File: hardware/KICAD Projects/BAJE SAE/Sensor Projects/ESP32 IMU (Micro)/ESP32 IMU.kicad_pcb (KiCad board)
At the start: 2 copper layers, 57.1 x 72 mm, 12 parts, among them J1 +5V, U1 BA50JC5T

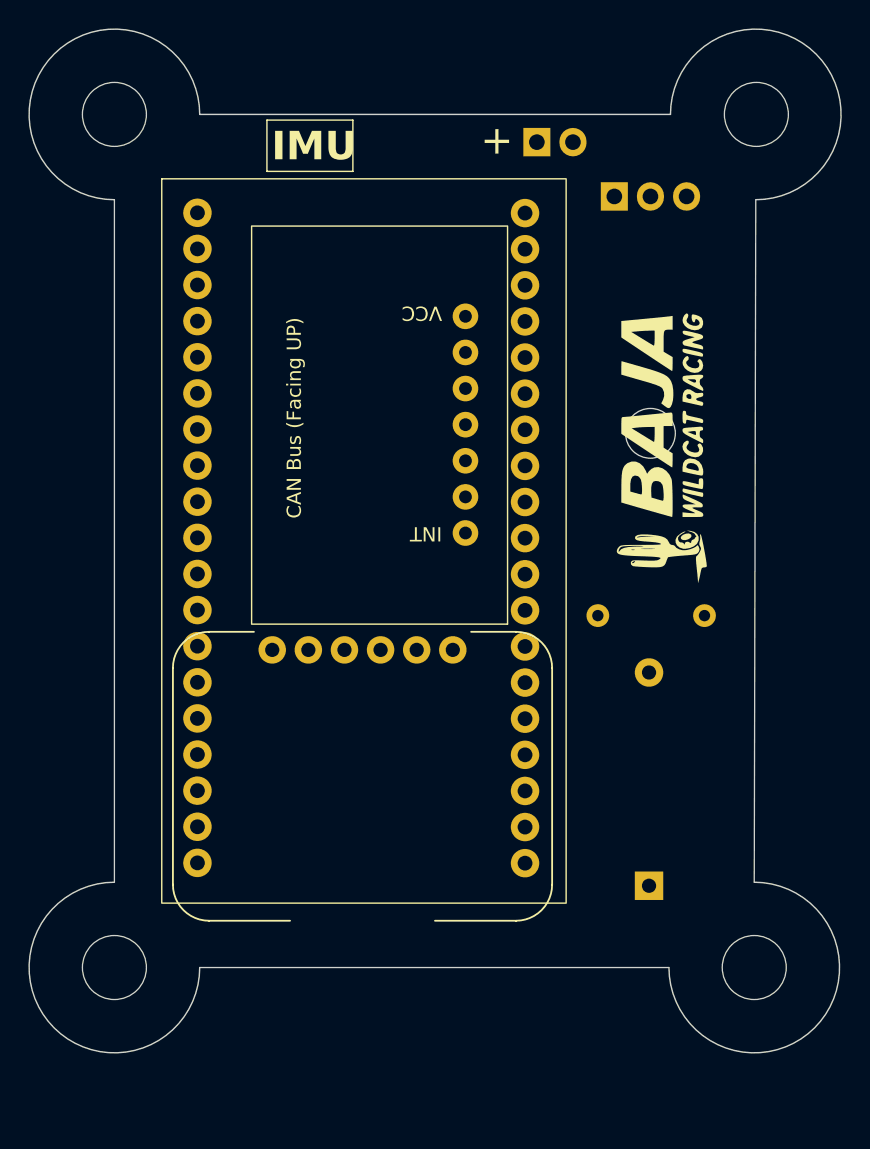
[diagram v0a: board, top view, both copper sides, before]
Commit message: Finished rough sketch of the ESP32 IMU Micro
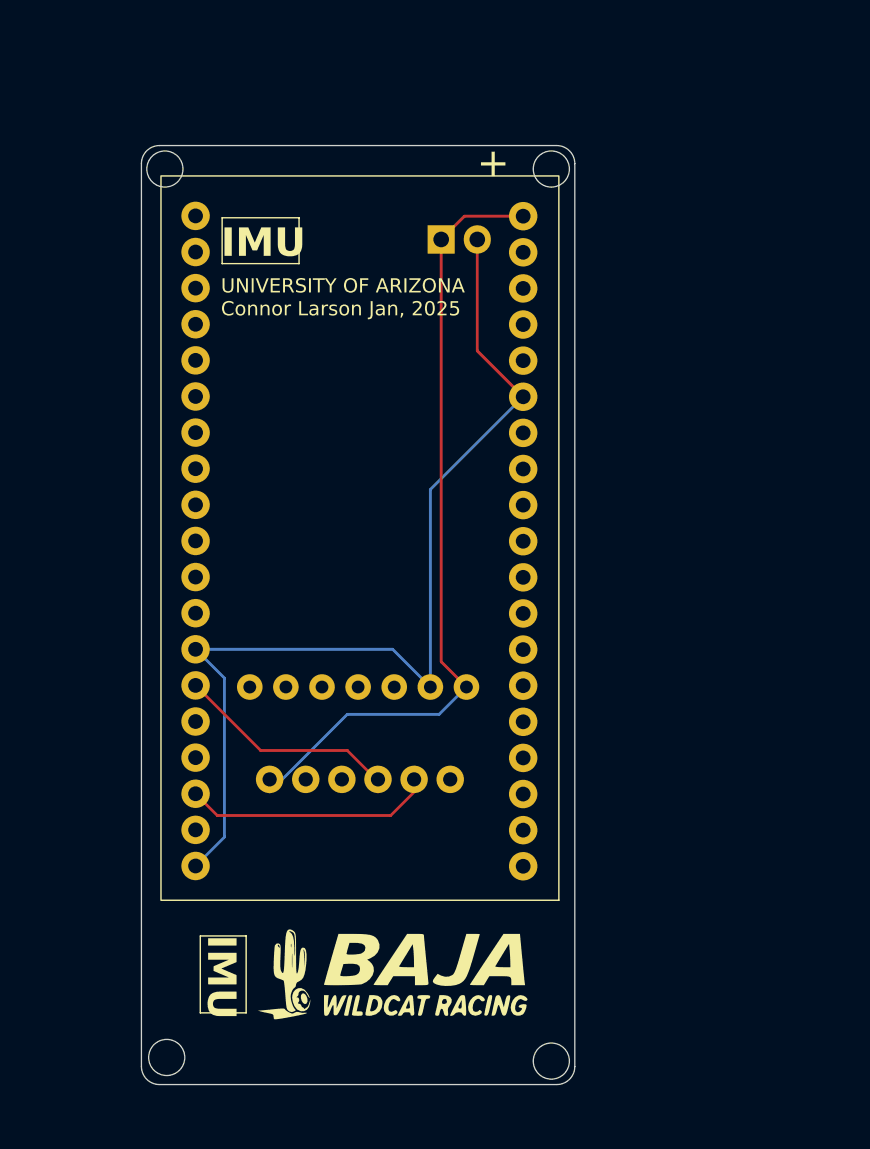
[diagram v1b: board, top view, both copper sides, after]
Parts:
- removed C1: .33u, Capacitor_THT:C_Axial_L3.8mm_D2.6mm_P7.50mm_Horizontal
- removed C2: 22u, Capacitor_THT:CP_Axial_L11.0mm_D8.0mm_P15.00mm_Horizontal
- removed REF** (x4): MountingHole_4.5mm, MountingHole:MountingHole_4.5mm
- removed U1: BA50JC5T, Package_TO_SOT_THT:TO-220-3_Horizontal_TabDown
- CAN Bus (Facing UP): moved to B.Cu
- UNIT_3: moved to B.Cu
- moved G*** 41.6 mm to (132.0, 118.0), turned to 0 degrees
- moved CAN Bus (Facing UP) 10.8 mm to (129.8, 80.0), turned to 90 degrees
- moved J1 9.60 mm to (136.4, 65.8)
- moved UNIT_3 9.11 mm to (129.7, 113.2), turned to 0 degrees
- moved UNIT_1 8.12 mm to (129.4, 91.4), turned to 180 degrees
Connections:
- J1 pad 1: Net-(J1-Pin_1) -> +5v
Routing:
- net GND: track 0.00 -> 70.1 mm
- net +5v: track 0.00 -> 55.6 mm
- net SCL: track 0.00 -> 16.7 mm
- net SDA: track 0.00 -> 16.4 mm
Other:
- board size 57.1 x 72 mm -> 30.5 x 66 mm
- board text added: "UNIVERSITY OF ARIZONA Connor Larson Jan, 2025"
- board text removed: "UNIVERSITY OF ARIZONA Connor Larson Nov, 2024"

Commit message: fixed issue that causes the whole pcb not to work
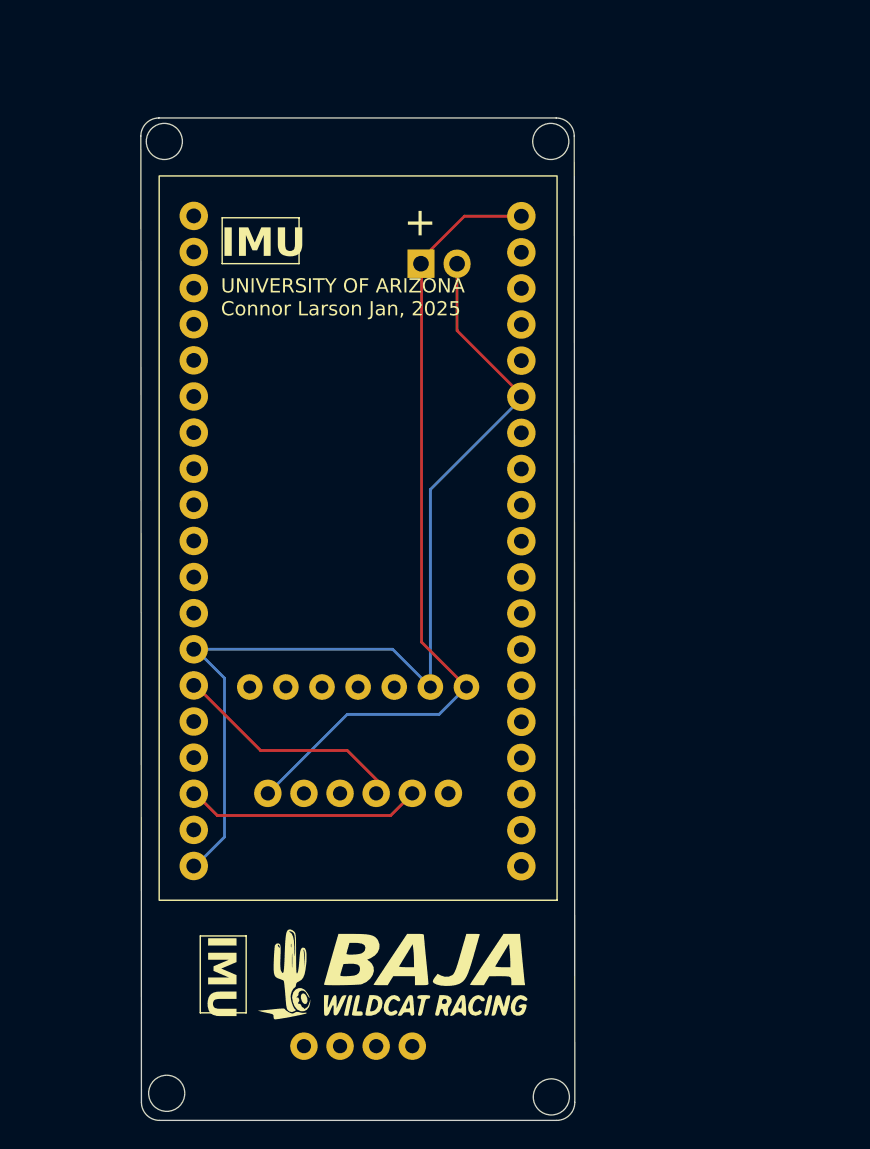
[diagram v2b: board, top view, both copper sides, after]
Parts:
- moved J1 2.22 mm to (135.0, 67.5)
- moved UNIT_3 0.99 mm to (129.5, 114.1)
- moved UNIT_1 0.13 mm to (129.3, 91.4)
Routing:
- net +5v: track 55.6 -> 56.7 mm
- net GND: track 70.1 -> 69.2 mm
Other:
- board size 30.5 x 66 mm -> 30.5 x 70.5 mm
